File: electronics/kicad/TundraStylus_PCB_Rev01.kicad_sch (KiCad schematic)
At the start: 11 parts, among them J1 CON_TPAD, J2 CON_MENU, J3 CON_TRIG, J4 CON_GRIP, SW1 TPAD, SW2 MENU, SW3 TRIG, SW4 GRIP

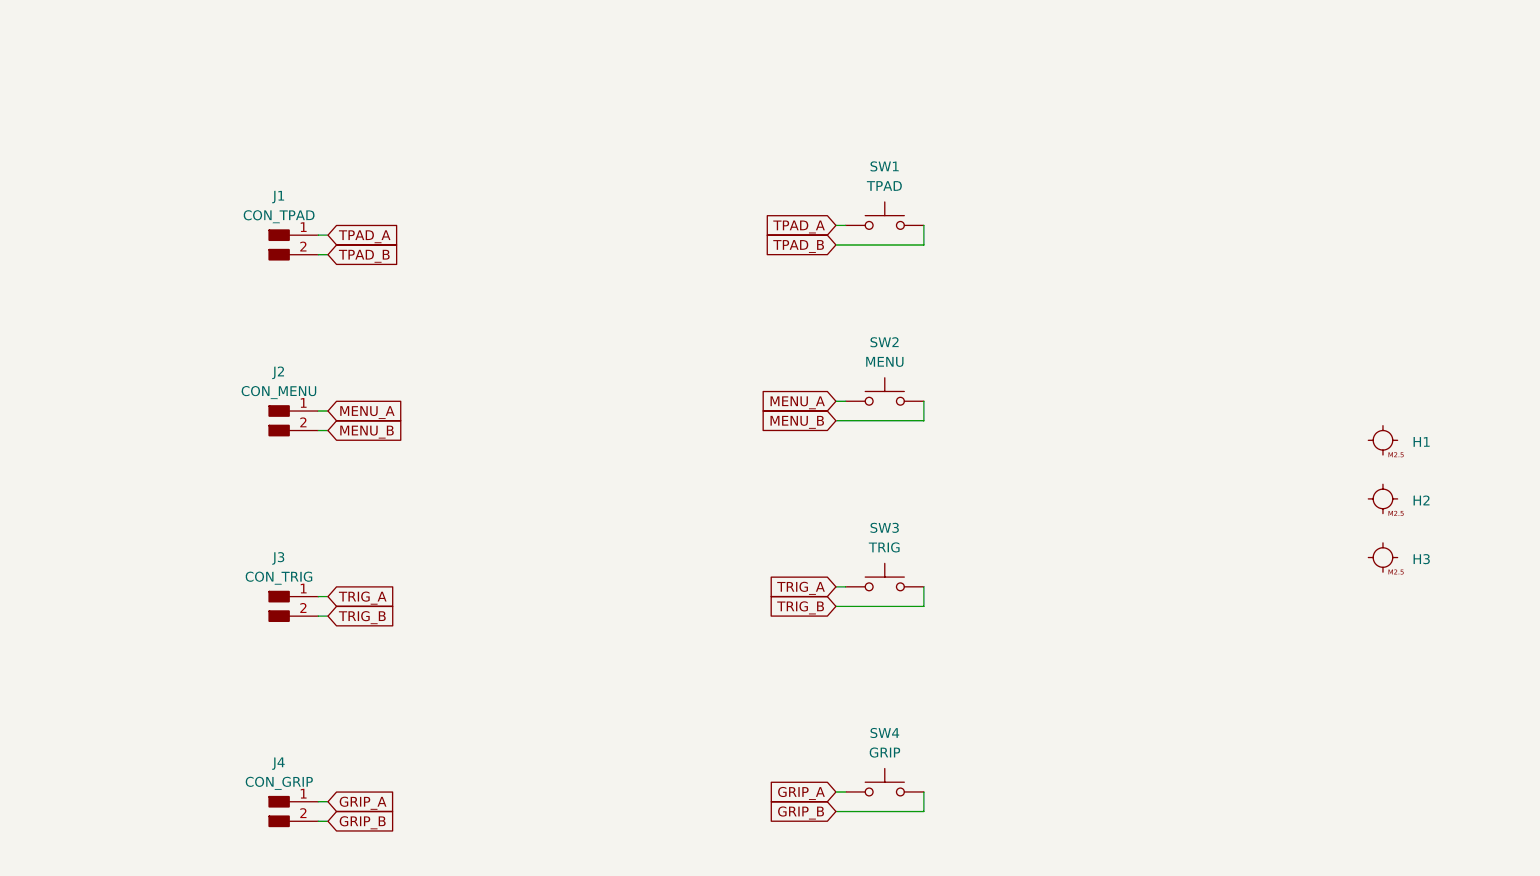
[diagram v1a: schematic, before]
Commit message: Add latest electronics design
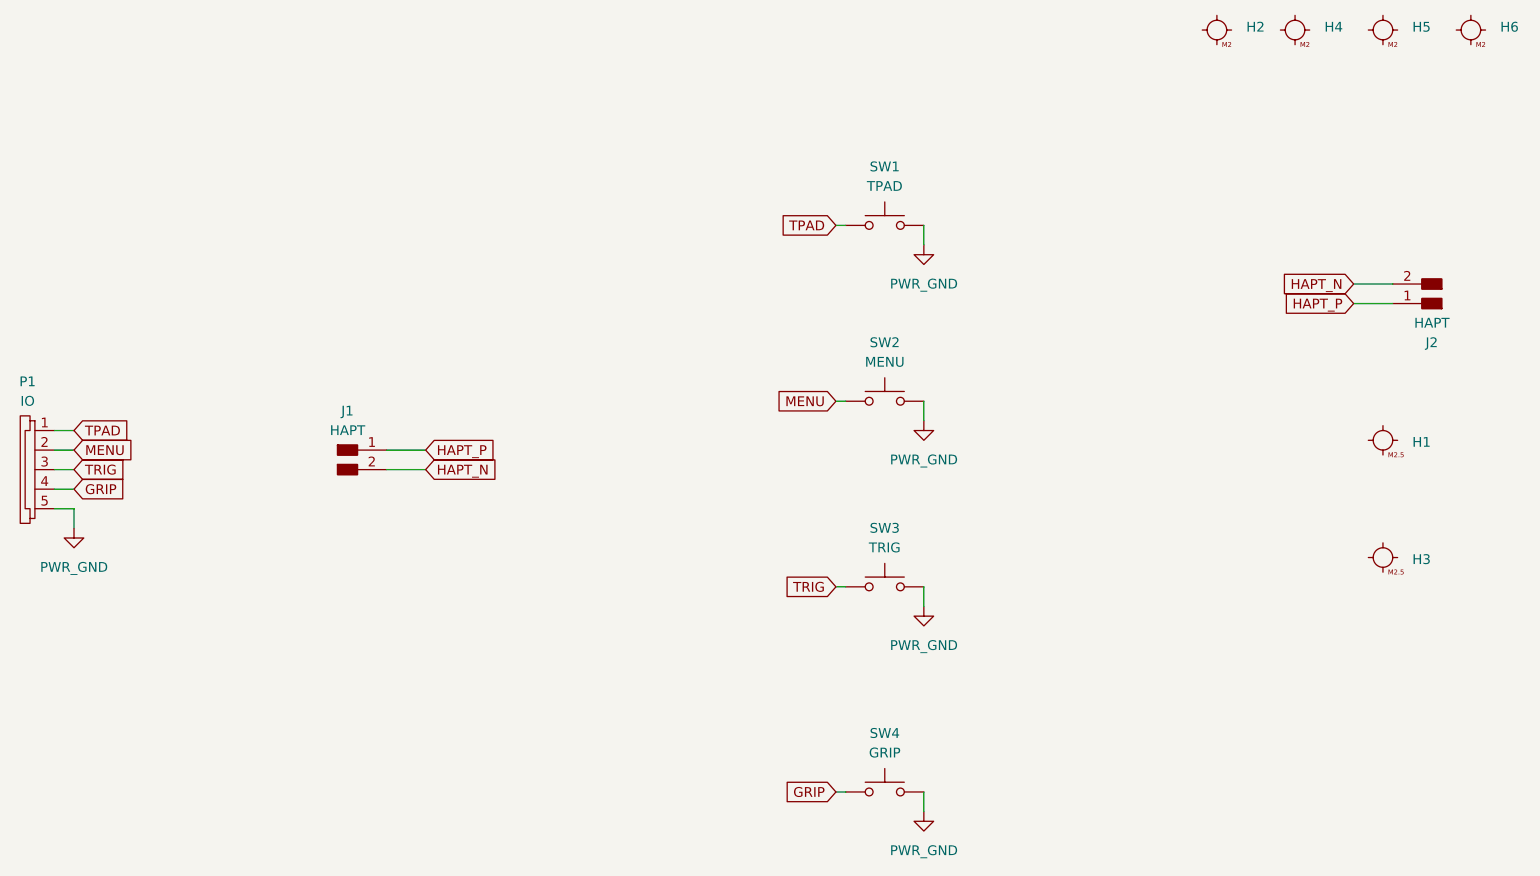
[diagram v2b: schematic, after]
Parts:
- removed H2: ~, fab:MountingHole_M2.5, symbol fab:MountingHole_M2.5
- removed J1: CON_TPAD, fab:PinHeader_1x02_P2.54mm_Horizontal_SMD, symbol fab:Conn_PinHeader_1x02_P2.54mm_Horizontal_SMD
- removed J2: CON_MENU, fab:PinHeader_1x02_P2.54mm_Horizontal_SMD, symbol fab:Conn_PinHeader_1x02_P2.54mm_Horizontal_SMD
- removed J3: CON_TRIG, fab:PinHeader_1x02_P2.54mm_Horizontal_SMD, symbol fab:Conn_PinHeader_1x02_P2.54mm_Horizontal_SMD
- removed J4: CON_GRIP, fab:PinHeader_1x02_P2.54mm_Horizontal_SMD, symbol fab:Conn_PinHeader_1x02_P2.54mm_Horizontal_SMD
- added H2, H4, H5, H6: ~, fab:MountingHole_M2, symbol fab:MountingHole_M2
- added J1, J2: HAPT, TundraIO:Conn_2pos_Plain, symbol fab:PinHeader_01x02_P2.54mm_Horizontal_SMD
- added P1: IO, TundraIO:Conn_FFC_1x05_P1mm_SideEntry_GCT_FFC3B11-05-T, symbol TundraIO:Conn_FFC_1x05_P1mm_SideEntry_GCT_FFC3B11-05-T
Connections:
- net MENU_B is gone; now on net PWR_GND: SW2.2
- net TPAD_B is gone; now on net PWR_GND: SW1.2
- net TRIG_B is gone; now on net PWR_GND: SW3.2
- net GRIP_A renamed GRIP
- net GRIP: now also P1.4
- net GRIP_B renamed PWR_GND
- net PWR_GND: now also P1.5
- net MENU_A renamed MENU
- net MENU: now also P1.2
- net TPAD_A renamed TPAD
- net TPAD: now also P1.1
- net TRIG_A renamed TRIG
- net TRIG: now also P1.3
- new net HAPT_N: J1.2 (Pin_2), J2.2 (Pin_2)
- new net HAPT_P: J1.1 (Pin_1), J2.1 (Pin_1)
